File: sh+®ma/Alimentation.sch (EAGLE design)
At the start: 17 parts, among them X1 87758-4016

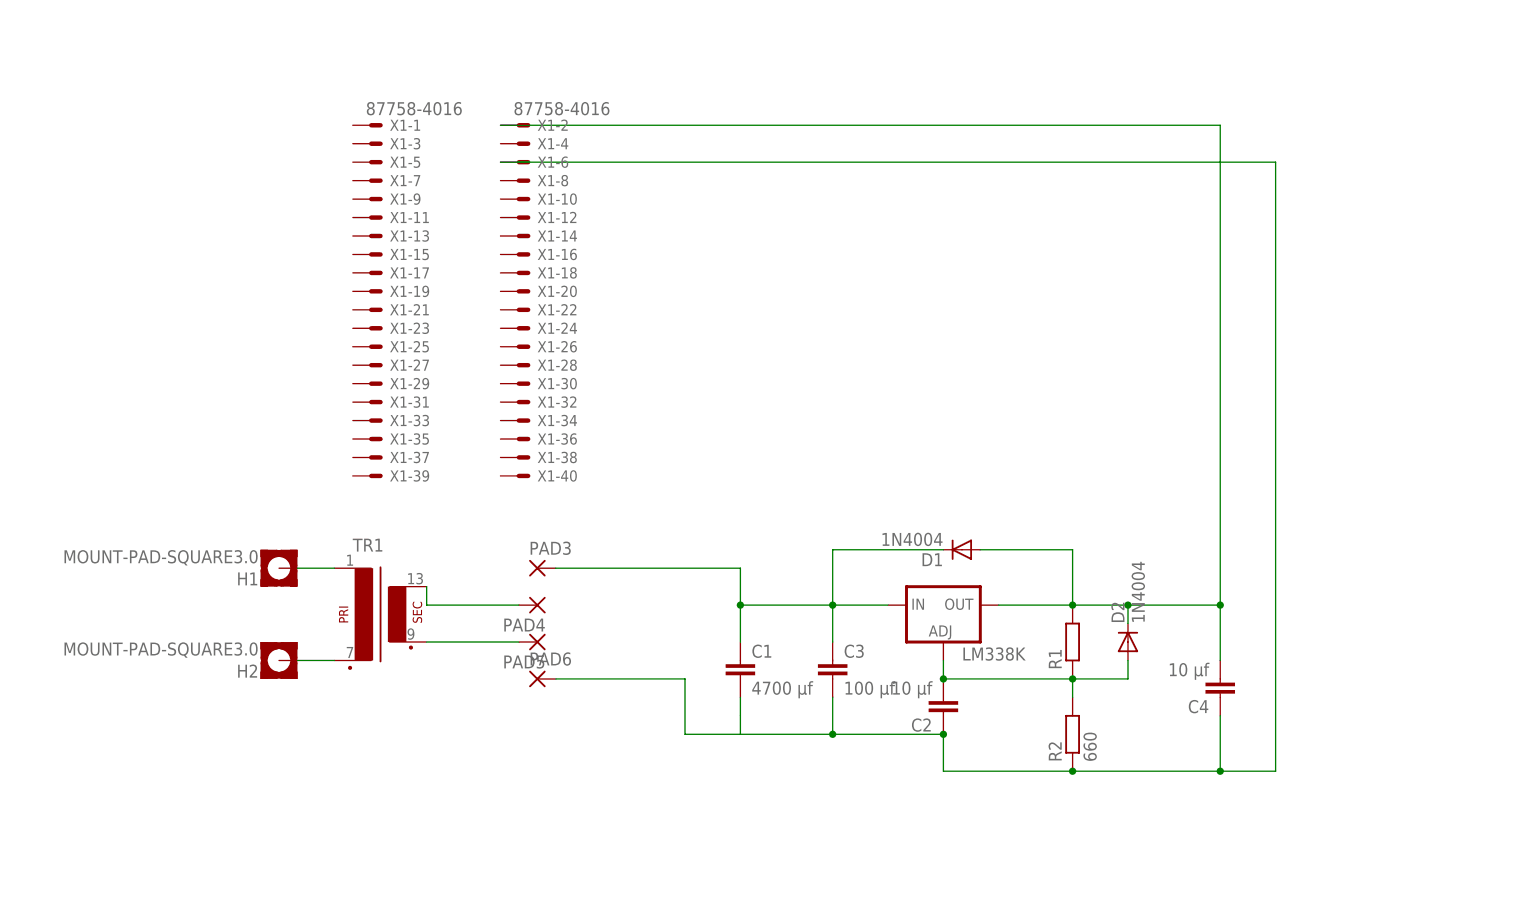
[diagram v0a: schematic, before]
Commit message: Carte mère (résolution problème transfo)
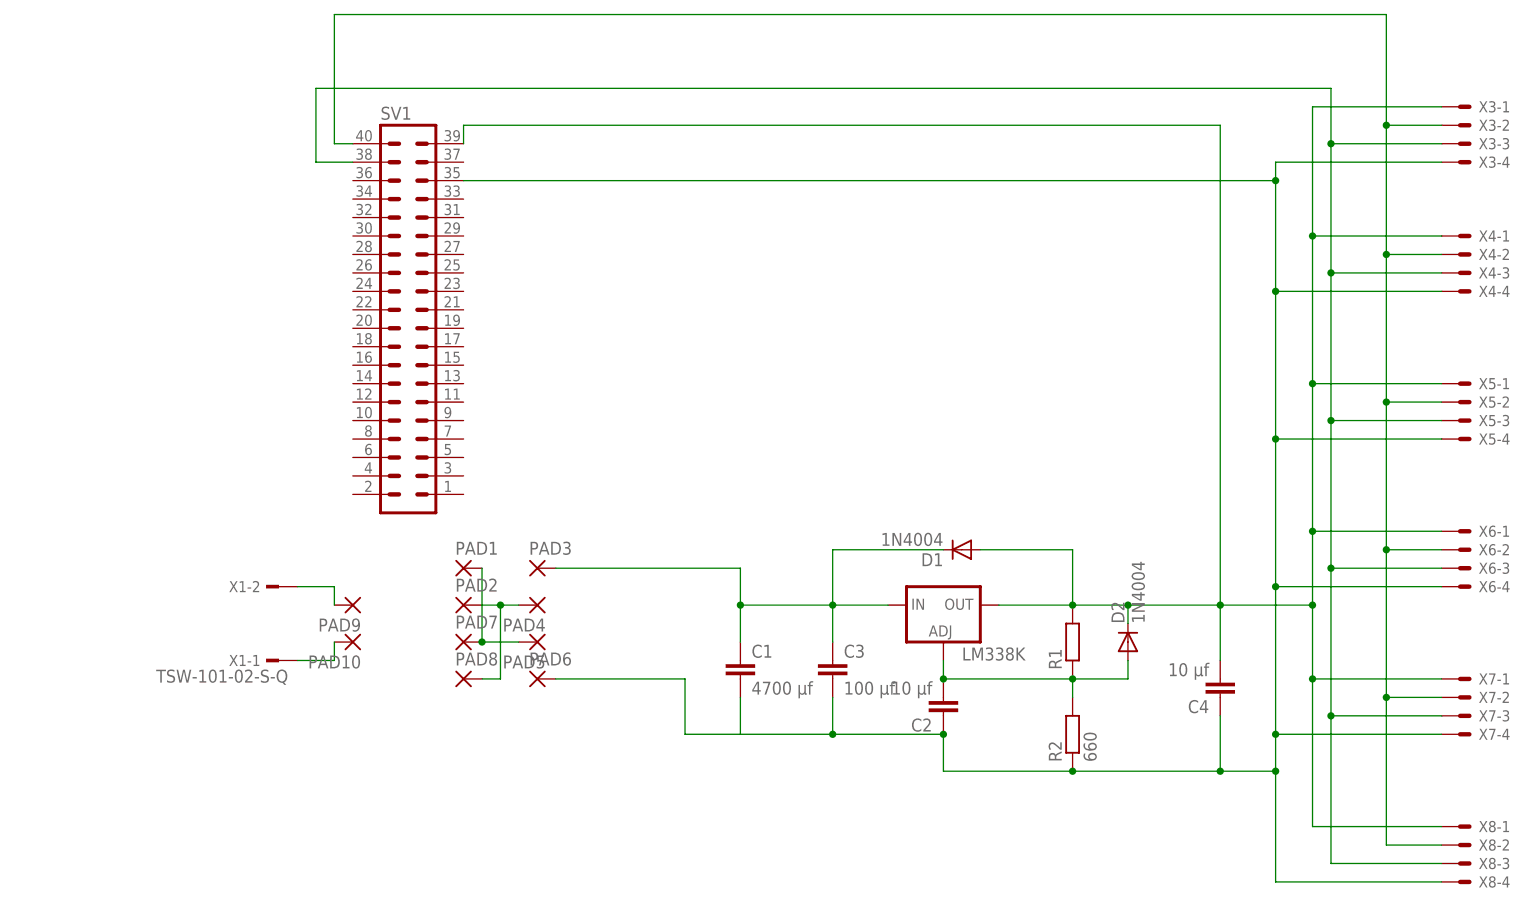
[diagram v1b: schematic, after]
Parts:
- removed H1, H2: MOUNT-PAD-SQUARE3.0, holes:MOUNT-PAD-SQUARE3.0
- removed TR1: (no value), trafo:EI54-1B
- added PAD1, PAD10, PAD2, PAD7, PAD8, PAD9: (no value), wirepad:2,54/1,1
- added SV1: (no value), con-lstb:MA20-2
- added X3, X4, X5, X6, X7, X8: (no value), con-molex:KK-156-4
- C2, C4: device rcl:C-EU050-075X075 -> capacitor-wima:C22/6
- X1: value 87758-4016 -> TSW-101-02-S-Q; device con-molex:87758-4016 -> con-samtec:TSW-101-02-S-Q
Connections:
- removed net N$8 (its old number): C4.2, D1.A, D2.C, LM338K.OUT, R1.2, X1-2.S
- new net N$10: C4.2, D1.A, D2.C, LM338K.OUT, R1.2, SV1.39, X3-1.S, X4-1.S, X5-1.S, X6-1.S, X7-1.S, X8-1.S
- new net N$7: SV1.38, X3-3.S, X4-3.S, X5-3.S, X6-3.S, X7-3.S, X8-3.S
- new net N$9: SV1.40, X3-2.S, X4-2.S, X5-2.S, X6-2.S, X7-2.S, X8-2.S
- net N$1: now also PAD9.P, X1-2.1; no longer PAD4.P, TR1.S4
- net N$2: now also PAD10.P, X1-1.1; no longer PAD5.P, TR1.S3
- net N$3: now also SV1.35, X3-4.S, X4-4.S, X5-4.S, X6-4.S, X7-4.S, X8-4.S; no longer X1-6.S
- net N$5: now also PAD2.P, PAD4.P, PAD8.P; no longer H1.MOUNT, TR1.P1
- net N$6: now also PAD1.P, PAD5.P, PAD7.P; no longer H2.MOUNT, TR1.P2
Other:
- moved on the sheet: X1-1, X1-2
